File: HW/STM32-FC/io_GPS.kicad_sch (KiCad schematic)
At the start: 4 parts, among them J2 2.54mm Male, Q1 S9013

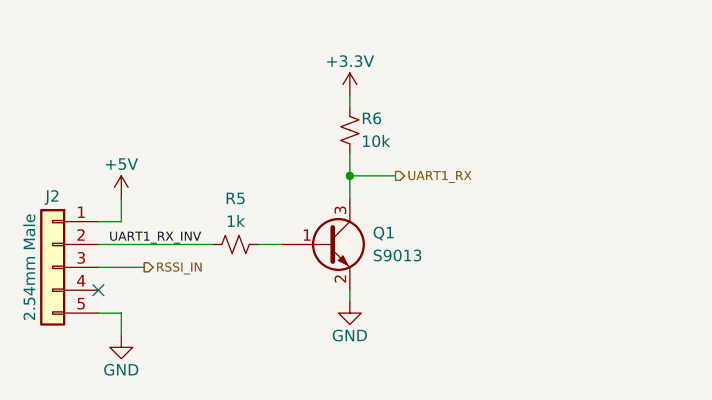
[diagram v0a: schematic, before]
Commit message: 250102:STM32F407VET
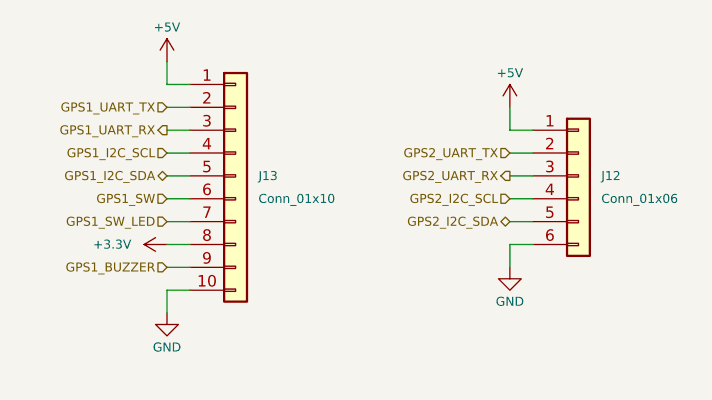
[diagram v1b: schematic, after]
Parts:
- removed J2: 2.54mm Male, Connector_PinHeader_2.54mm:PinHeader_1x03_P2.54mm_Vertical, symbol Connector_Generic:Conn_01x05
- removed Q1: S9013, digikey-footprints:SOT-23-3, symbol Device:Q_NPN_BEC
- removed R5: 1k, Resistor_SMD:R_0402_1005Metric, symbol Device:R_Small_US
- removed R6: 10k, Resistor_SMD:R_0402_1005Metric, symbol Device:R_Small_US
- added J12: Conn_01x06, Connectors_JST:JST_GH_BM06B-GHS-TBT_06x1.25mm_Straight, symbol Connector_Generic:Conn_01x06
- added J13: Conn_01x10, Connectors_JST:JST_GH_BM06B-GHS-TBT_06x1.25mm_Straight, symbol Connector_Generic:Conn_01x10
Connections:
- net +3.3V: now also J13.8 (Pin_8)
- net +5V: now also J12.1 (Pin_1), J13.1 (Pin_1)
- net GND: now also J12.6 (Pin_6), J13.10 (Pin_10)
- new net GPS1_BUZZER: J13.9 (Pin_9)
- new net GPS1_I2C_SCL: J13.4 (Pin_4)
- new net GPS1_I2C_SDA: J13.5 (Pin_5)
- new net GPS1_SW: J13.6 (Pin_6)
- new net GPS1_SW_LED: J13.7 (Pin_7)
- new net GPS1_UART_RX: J13.3 (Pin_3)
- new net GPS1_UART_TX: J13.2 (Pin_2)
- new net GPS2_I2C_SCL: J12.4 (Pin_4)
- new net GPS2_I2C_SDA: J12.5 (Pin_5)
- new net GPS2_UART_RX: J12.3 (Pin_3)
- new net GPS2_UART_TX: J12.2 (Pin_2)
- no-connect marks 1 -> 0
